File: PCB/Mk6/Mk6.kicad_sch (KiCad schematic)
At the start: 1 part, among them J28 EXTENSION

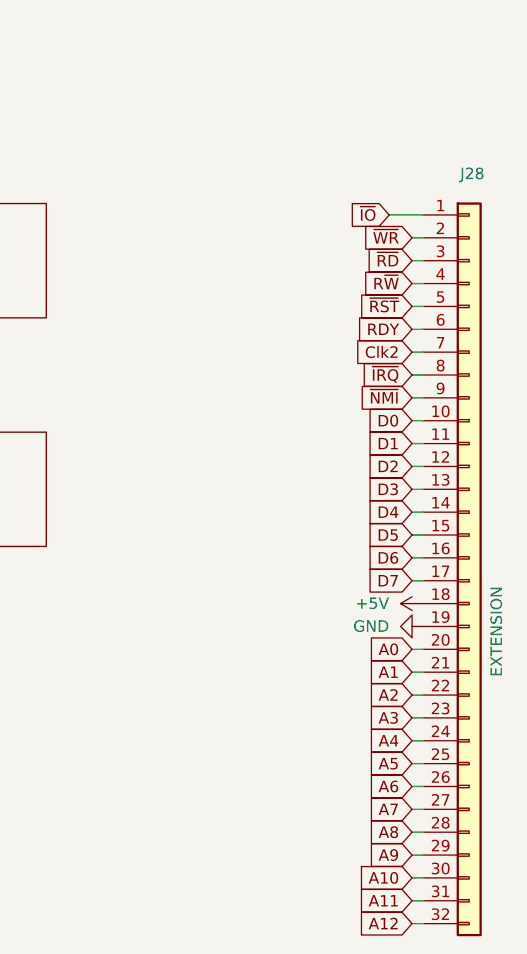
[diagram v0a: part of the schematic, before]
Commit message: save
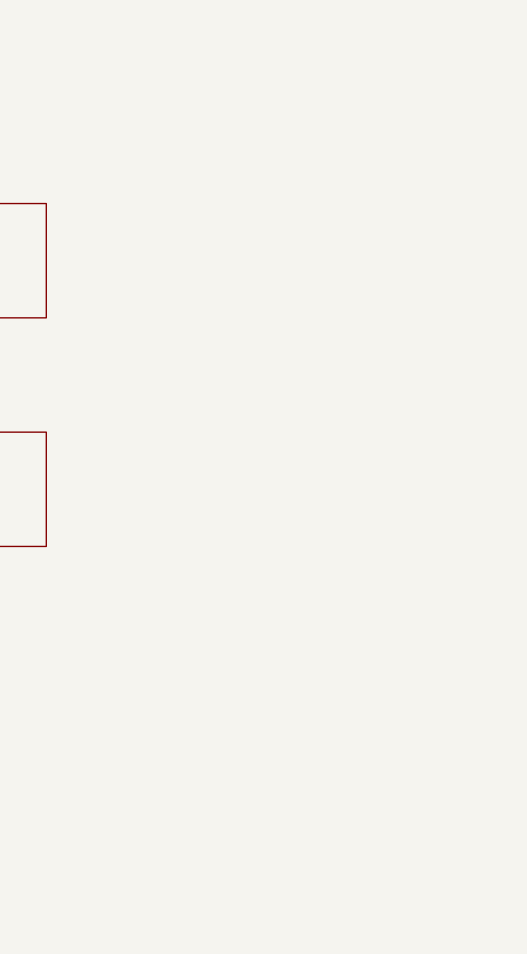
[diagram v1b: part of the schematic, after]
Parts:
- removed J28: EXTENSION, Connector_PinSocket_2.54mm:PinSocket_1x32_P2.54mm_Vertical, symbol Connector_Generic:Conn_01x32
